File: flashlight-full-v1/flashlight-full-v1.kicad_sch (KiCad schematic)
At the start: 99 parts, among them J1 USB_C_Receptacle, J2 ST-LINK, J3 IO1, J4 IO2, J5 SYS, J6 GND, Q1 2N7002H, Q2 2N7002H, Q3 2N7002H, SW1 RESET, SW2 BOOT, U1 BQ25185DLHR, U2 STM32L151C8Tx, U3 MMA8452QR1, U4 MCP1703Ax-120xxTT, U5 MCP1703Ax-120xxTT, U6 SMF05CT1G

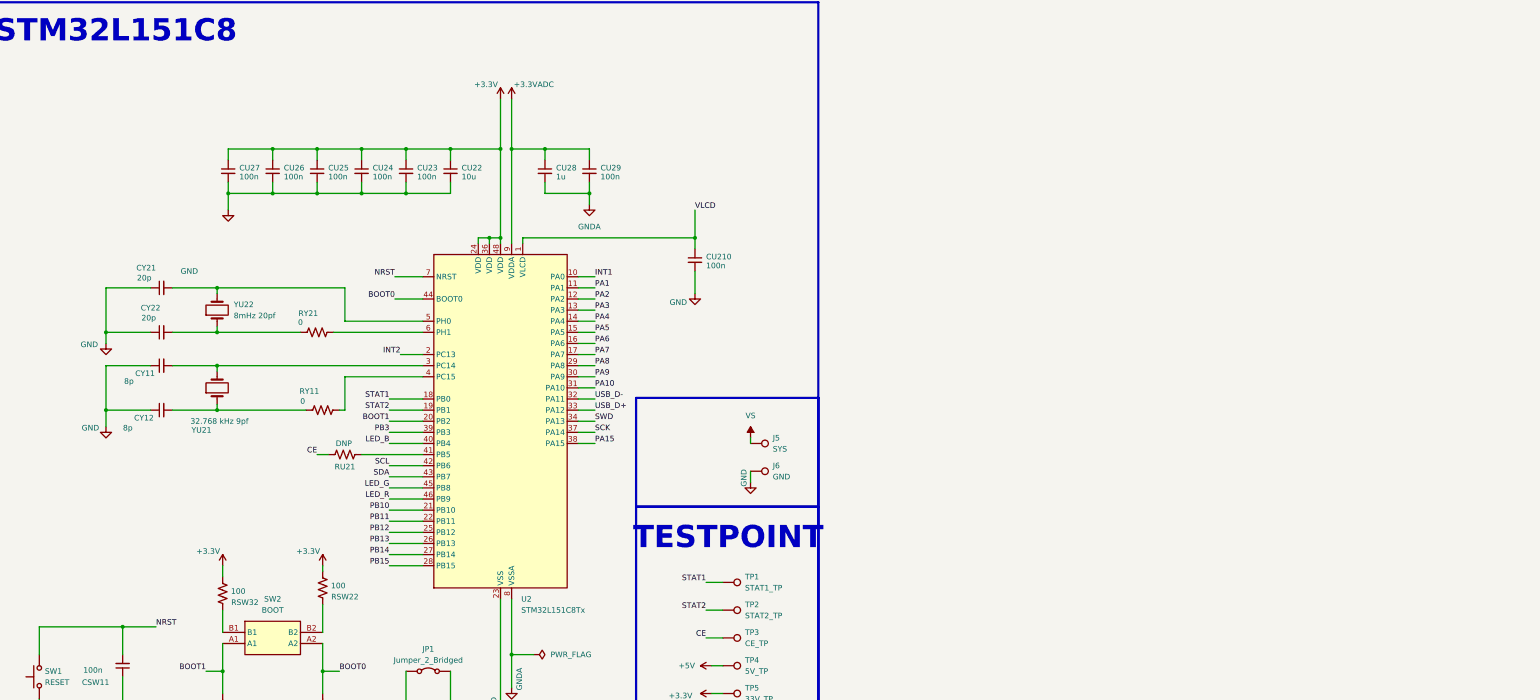
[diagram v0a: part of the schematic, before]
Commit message: full init
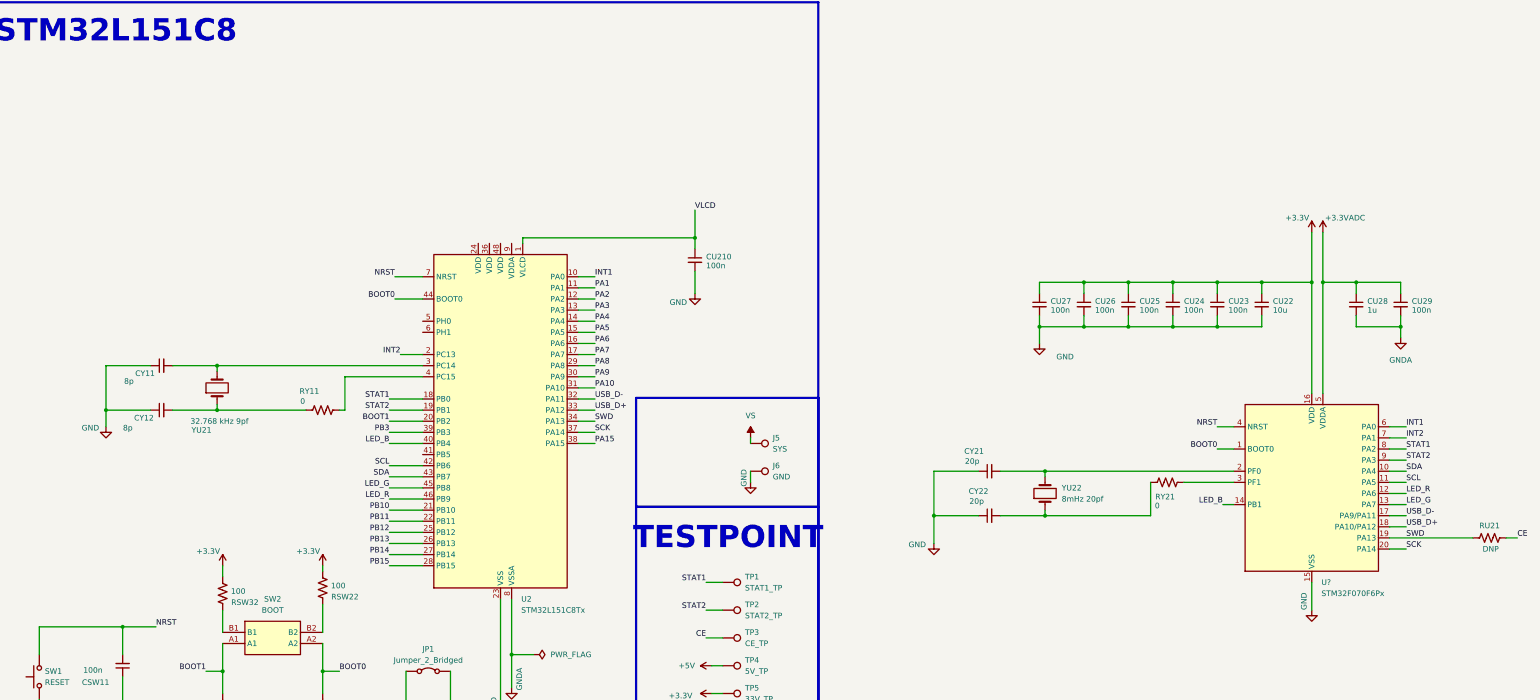
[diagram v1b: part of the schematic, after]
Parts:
- added U?: STM32F070F6Px, Package_SO:TSSOP-20_4.4x6.5mm_P0.65mm, symbol MCU_ST_STM32F0:STM32F070F6Px
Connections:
- net +3.3V: now also U?.16 (VDD); no longer U2.24 (VDD), U2.36 (VDD), U2.48 (VDD)
- net +3.3VADC: now also U?.5 (VDDA); no longer U2.9 (VDDA)
- net BOOT0: now also U?.1 (BOOT0)
- net GND: now also U?.15 (VSS)
- net INT1: now also U?.6 (PA0)
- net INT2: now also U?.7 (PA1)
- net LED_B: now also U?.14 (PB1)
- net LED_G: now also U?.13 (PA7)
- net LED_R: now also U?.12 (PA6)
- net NRST: now also U?.4 (NRST)
- net SCK: now also U?.20 (PA14)
- net SCL: now also U?.11 (PA5)
- net SDA: now also U?.10 (PA4)
- net STAT1: now also U?.8 (PA2)
- net STAT2: now also U?.9 (PA3)
- net SWD: now also RU21.1, U?.19 (PA13)
- net USB_D+: now also U?.18 (PA10/PA12)
- net USB_D-: now also U?.17 (PA9/PA11)
- net at RY21.1: now also U?.3 (PF1); no longer U2.6 (PH1)
- net at U2.41 (PB5): no longer RU21.1
- net at CY21.2, YU22.2: now also U?.2 (PF0); no longer U2.5 (PH0)
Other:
- moved on the sheet: CU22, CU23, CU24, CU25, CU26, CU27, CU28, CU29, CY21, CY22, RU21, RY21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
